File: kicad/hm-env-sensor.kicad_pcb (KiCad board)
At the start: 2 copper layers, 40 x 79 mm, 65 parts, among them Q1 Q12MHz/20pF/10ppm/4P/3.2x2.5mm, Q2 BC817-40(SOT23), Q3 BC817-40(SOT23), U1 BL4054B-42TPRN(SOT23-5), U2 CH340T(SSOP20W), U3 SY8089AAAC(SOT23-5), U4 BAT54C(SOT23-3), U5 ESP-WROOM-32, U6 BQ27441-G1, U7 BME280

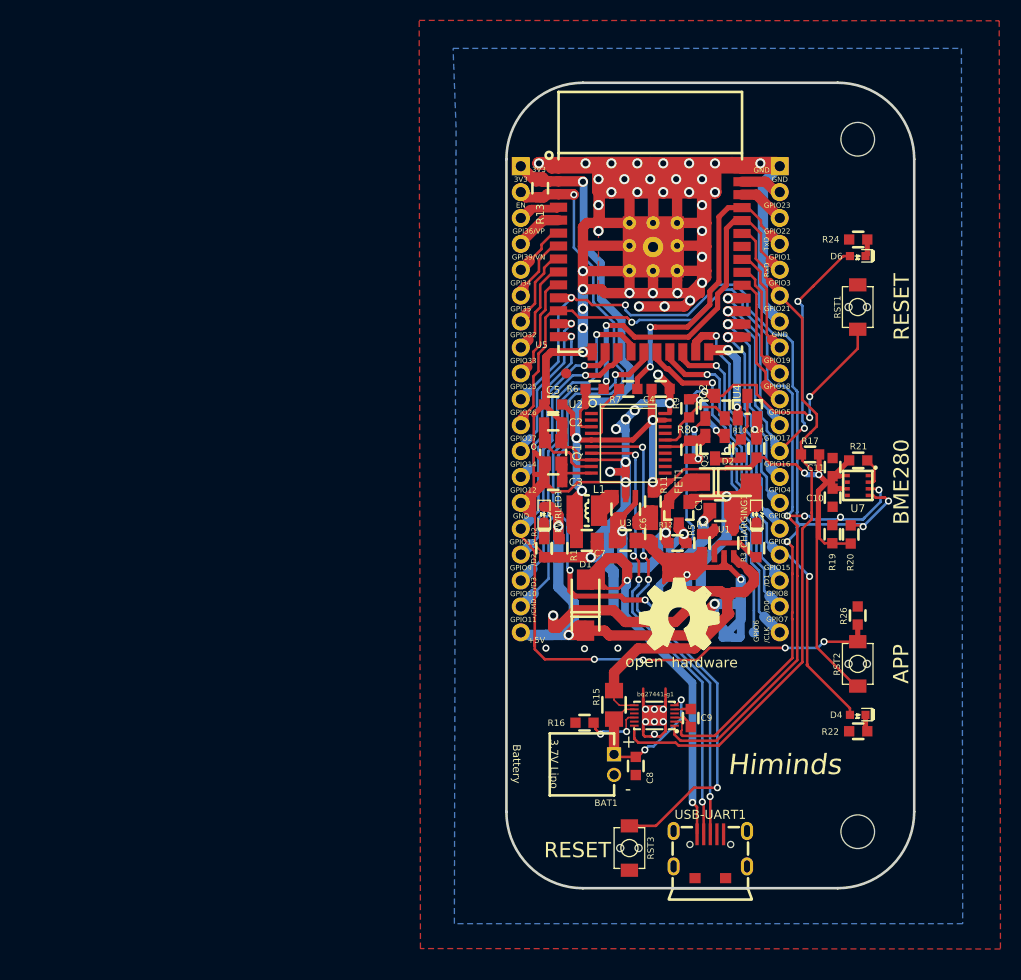
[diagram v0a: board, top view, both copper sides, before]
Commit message: Rev B updates
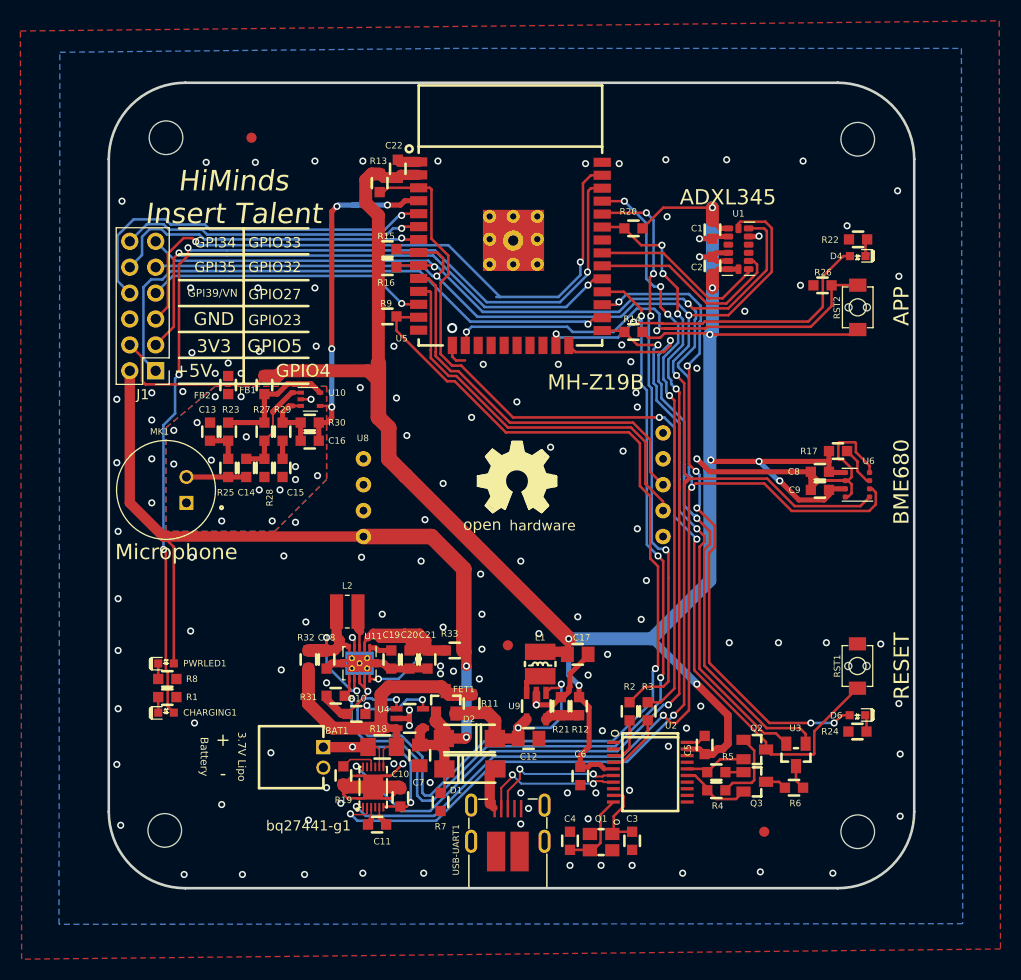
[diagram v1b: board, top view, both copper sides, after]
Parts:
- removed the ? at (146.3, 116.8)
- removed D_Com1, GND1: TESTPAD, OLIMEX_Other-FP:TESTPAD_40-ROUND
- removed EXT1, EXT2: HN1x19, OLIMEX_Connectors-FP:HN1x19
- removed RST3: IT-1185AU2-160G-G-TR, OLIMEX_Buttons-FP:IT1185AU2_V2
- added ?: , hm-env-sensor:LOGO_OPENHARDWARE_8x8, F.Cu at (130.4, 103.4)
- added C12: 47uF/6.3V/20%/X5R/C0805, OLIMEX_RLC-FP:C_0805_5MIL_DWS, F.Cu at (131.6, 128.5)
- added C13: 100nF/50V/20%/Y5V/C0603, OLIMEX_RLC-FP:C_0603_5MIL_DWS, F.Cu at (100.3, 98.4)
- added C14: 10nF/50V/20%/Y5V/C0603, OLIMEX_RLC-FP:C_0603_5MIL_DWS, F.Cu at (103.9, 102.0)
- added C15: 10uF/C0603, OLIMEX_RLC-FP:C_0603_5MIL_DWS, F.Cu at (107.4, 102.0)
- added C16: 100pF/C0603, OLIMEX_RLC-FP:C_0603_5MIL_DWS, F.Cu at (110.1, 99.3)
- added C17: 47uF/6.3V/20%/X5R/C0805, OLIMEX_RLC-FP:C_0805_5MIL_DWS, F.Cu at (136.4, 120.3)
- added C18: 10uF/6.3V/X7R/C0603, OLIMEX_RLC-FP:C_0603_5MIL_DWS, F.Cu at (111.8, 120.8)
- added C19: 1uF/6.3V/X7R/C0603, OLIMEX_RLC-FP:C_0603_5MIL_DWS, F.Cu at (118.1, 120.8)
- added C20: 10uF/6.3V/X7R/C0603, OLIMEX_RLC-FP:C_0603_5MIL_DWS, F.Cu at (119.9, 120.8)
- added C21: 10uF/6.3V/X7R/C0603, OLIMEX_RLC-FP:C_0603_5MIL_DWS, F.Cu at (121.7, 120.8)
- added C22: 10uF/6.3V/X7R/C0603, OLIMEX_RLC-FP:C_0603_5MIL_DWS, F.Cu at (118.7, 72.6)
- added FB1: Ferrite_Bead_Small, OLIMEX_RLC-FP:L_0603_5MIL_DWS, F.Cu at (105.7, 93.9)
- added FB2: Ferrite_Bead_Small, OLIMEX_RLC-FP:L_0603_5MIL_DWS, F.Cu at (102.1, 93.9)
- added FID1: Fiducial, OLIMEX_Other-FP:Fiducial1x3, F.Cu at (104.4, 69.6)
- added FID2: Fiducial, OLIMEX_Other-FP:Fiducial1x3, F.Cu at (154.7, 137.7)
- added J1: Conn_02x06_Odd_Even, Connector_PinHeader_2.54mm:PinHeader_2x06_P2.54mm_Vertical, F.Cu at (95.0, 92.5)
- added L2: LPS3015-222ML, Inductor_SMD:L_Wuerth_MAPI-3015, F.Cu at (113.8, 116.1)
- added MK1: Microphone, hm-env-sensor:MIC_CMA-4544PF-W, F.Cu at (96.0, 104.1)
- added MountingHole*: Mounting_hole_3.3mm, OLIMEX_Other-FP:Mounting_hole_3.3mm, F.Cu at (98.9, 56.0)
- added MountingHole*: Mounting_hole_3.3mm, OLIMEX_Other-FP:Mounting_hole_3.3mm, F.Cu at (98.8, 124.0)
- added R18: 0.01/1%/R1206, OLIMEX_RLC-FP:R_1206_5MIL_DWS, F.Cu at (117.2, 129.3)
- added R23: 1k/R0603, OLIMEX_RLC-FP:R_0603_5MIL_DWS, F.Cu at (102.1, 98.4)
- added R25: 1k/R0603, OLIMEX_RLC-FP:R_0603_5MIL_DWS, F.Cu at (102.1, 102.0)
- added R27: 1M/R0603, OLIMEX_RLC-FP:R_0603_5MIL_DWS, F.Cu at (105.7, 98.4)
- added R28: 1M/R0603, OLIMEX_RLC-FP:R_0603_5MIL_DWS, F.Cu at (105.7, 102.0)
- added R29: 1k/R0603, OLIMEX_RLC-FP:R_0603_5MIL_DWS, F.Cu at (107.4, 98.4)
- added R30: 20k/R0603, OLIMEX_RLC-FP:R_0603_5MIL_DWS, F.Cu at (110.1, 97.5)
- added R31: 10k, OLIMEX_RLC-FP:R_0603_5MIL_DWS, F.Cu at (112.6, 124.3)
- added R32: NA/R0603, OLIMEX_RLC-FP:R_0603_5MIL_DWS, F.Cu at (110.0, 120.8)
- added R33: NA/R0603, OLIMEX_RLC-FP:R_0603_5MIL_DWS, F.Cu at (124.3, 119.9)
- added U10: MAX4466, Package_TO_SOT_SMD:SOT-353_SC-70-5, F.Cu at (110.2, 95.2)
- added U11: TPS61202DRC, Package_SON:Texas_S-PVSON-N10_ThermalVias, F.Cu at (115.0, 121.1)
- added U8: MH-Z19B, hm-env-sensor:MH-Z19B, F.Cu at (130.0, 96.0)
- added U9: SY8089AAAC(SOT23-5), OLIMEX_Regulators-FP:SOT-23-5, F.Cu at (132.3, 125.3)
- C1: value 47uF/6.3V/20%/X5R/C0805 -> 4.7uF/50V/20%/Y5V/C0603; footprint OLIMEX_RLC-FP:C_0805_5MIL_DWS -> OLIMEX_RLC-FP:C_0603_5MIL_DWS
- C10: value 100nF/50V/20%/Y5V/C0603 -> 1.0uF/16V/10%/Y5V/C0603
- C11: value 100nF/50V/20%/Y5V/C0603 -> 0.47uF/50V/20%/Y5V/C0603
- C2: value 27pF/50V/5%/C0G/C0603 -> 100nF/50V/20%/Y5V/C0603
- C4: value 22uF/6.3V/20%/X5R/C0603 -> 27pF/50V/5%/C0G/C0603
- C5: value 100nF/50V/20%/Y5V/C0603 -> 22uF/6.3V/20%/X5R/C0603
- C6: value 47uF/6.3V/20%/X5R/C0805 -> 100nF/50V/20%/Y5V/C0603; footprint OLIMEX_RLC-FP:C_0805_5MIL_DWS -> OLIMEX_RLC-FP:C_0603_5MIL_DWS
- C8: value 1.0uF/16V/10%/Y5V/C0603 -> 100nF/50V/20%/Y5V/C0603
- C9: value 0.47uF/50V/20%/Y5V/C0603 -> 100nF/50V/20%/Y5V/C0603
- PWRLED1: value LED/RED/0603 -> LED/GREEN/0603
- R1: value 10k/R0603 -> 330/R0603
- R10: value 220R/R0603 -> 2.2k/R0603
- R11: value 4.99k/1%/R0603 -> NA/R0603
- R12: value 1.1k/1%/R0603 -> 4.99k/1%/R0603
- R15: value 0.01/1%/R1206 -> 4.7k/R0603; footprint OLIMEX_RLC-FP:R_1206_5MIL_DWS -> OLIMEX_RLC-FP:R_0603_5MIL_DWS
- R16: value 10k/R0603 -> 4.7k/R0603
- R19: value 4.7k/R0603 -> 10k/R0603
- R2, R3: value 2.2k/R0603 -> 220R/R0603
- R21: value 4.7k/R0603 -> 1.1k/1%/R0603
- R4: value 2.2k/R0603 -> 1k/R0603
- R5: value NA/R0603 -> 1k/R0603
- R7: value 220R/R0603 -> 10k/R0603
- R8: value 1k/R0603 -> 4.7k/R0603
- R9: value 1k/R0603 -> 10k/R0603
- U1: value BL4054B-42TPRN(SOT23-5) -> ADXL345; footprint OLIMEX_IC-FP:SOT-23-5 -> Package_LGA:LGA-14_3x5mm_P0.8mm_LayoutBorder1x6y
- U3: value SY8089AAAC(SOT23-5) -> BAT54C(SOT23-3); footprint OLIMEX_Regulators-FP:SOT-23-5 -> OLIMEX_Diodes-FP:SOT23-3
- U4: value BAT54C(SOT23-3) -> BL4054B-42TPRN(SOT23-5); footprint OLIMEX_Diodes-FP:SOT23-3 -> OLIMEX_IC-FP:SOT-23-5
- U6: value BQ27441-G1 -> BME680; footprint sparkfun-battery-babysitter:PDSO-N12 -> Package_LGA:Bosch_LGA-8_3x3mm_P0.8mm_ClockwisePinNumbering
- U7: value BME280 -> BQ27441-G1; footprint SparkFun_BME280_Breakout_v10:BME280_LGA -> hm-env-sensor:PDSO-N12
- USB-UART1: footprint OLIMEX_Connectors-FP:USB-MICRO_MISB-SWMM-5B_LF -> hm-env-sensor:USB_Micro_B_Male_UJ2-MIBH-4-SMT-TR
- moved CHARGING1 61.1 mm to (96.0, 126.0), turned to 0 degrees
- moved C11 56.8 mm to (116.7, 137.0), turned to 180 degrees
- moved U7 56.0 mm to (116.3, 133.3)
- moved R8 55.9 mm to (96.1, 122.7), turned to 180 degrees
- moved R19 53.5 mm to (113.4, 132.1), turned to 90 degrees
- moved C10 51.6 mm to (119.0, 134.3), turned to 90 degrees
- moved R15 49.9 mm to (117.7, 80.5), turned to 180 degrees
- moved R16 48.7 mm to (117.7, 82.3), turned to 180 degrees
- moved R24 48.3 mm to (163.8, 127.8)
- moved R22 48.2 mm to (163.9, 79.6)
- moved R10 45.8 mm to (114.7, 126.1), turned to 180 degrees
- moved C4 45.2 mm to (135.6, 138.6), turned to 90 degrees
- moved U4 45.1 mm to (119.9, 126.6), turned to 180 degrees
- moved D6 45.0 mm to (163.8, 126.2)
- moved D4 45.0 mm to (163.9, 81.2)
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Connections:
- net /+5V_USB renamed /Power and charger/+5V_USB
- net Net-(U2-Pad6) renamed /USB2UART/D+
- net Net-(U2-Pad7) renamed /USB2UART/D-
- BAT1 pad 1: /BATTERY_IN -> /BATTERY
- C1 pad 1: +5V -> +3V3
- C10 pad 1: +3V3 -> /BATTERY
- C11 pad 1: +3V3 -> Net-(C11-Pad1)
- C2 pad 1: Net-(C2-Pad1) -> +3V3
- C4 pad 1: +3V3 -> Net-(C4-Pad1)
- C6 pad 1: Net-(C6-Pad1) -> +3V3
- C7 pad 1: +3V3 -> +5V
- C8 pad 1: /BATTERY_IN -> +3V3
- C9 pad 1: Net-(C9-Pad1) -> +3V3
- CHARGING1 pad 2: +5V -> /GPIO22
- D2 pad 1: Net-(C6-Pad1) -> Net-(C12-Pad1)
- FET1 pad 2: Net-(C6-Pad1) -> Net-(C12-Pad1)
- FET1 pad 3: V_BATT -> /AFTER_BAT_SENSOR
- Q1 pad 1: Net-(C2-Pad1) -> Net-(C3-Pad1)
- Q1 pad 2: Net-(C3-Pad1) -> Net-(C4-Pad1)
- R1 pad 1: +5V -> GND
- R1 pad 2: GND -> Net-(CHARGING1-Pad1)
- R10 pad 1: Net-(Q3-Pad3) -> Net-(R10-Pad1)
- R10 pad 2: /D_Com -> GND
- R11 pad 1: Net-(R11-Pad1) -> /AFTER_BAT_SENSOR
- R11 pad 2: +3V3 -> Net-(C12-Pad1)
- R12 pad 1: Net-(R11-Pad1) -> Net-(R12-Pad1)
- R12 pad 2: GND -> +3V3
- R15 pad 1: V_BATT -> /GPIO32
- R15 pad 2: /BATTERY_IN -> +3V3
- R16 pad 1: GND -> /GPIO33
- R16 pad 2: Net-(R16-Pad2) -> +3V3
- R17 pad 1: /GPIO21 -> Net-(R17-Pad1)
- R19 pad 1: /GPIO27 -> GND
- R19 pad 2: +3V3 -> Net-(R19-Pad2)
- R2 pad 1: Net-(PWRLED1-Pad1) -> Net-(R2-Pad1)
- R2 pad 2: GND -> /GPIO3
- R20 pad 1: /GPIO26 -> /GPIO21
- R21 pad 1: Net-(R21-Pad1) -> Net-(R12-Pad1)
- R21 pad 2: +3V3 -> GND
- R3 pad 1: Net-(CHARGING1-Pad1) -> Net-(R3-Pad1)
- R3 pad 2: Net-(R3-Pad2) -> /GPIO1
- R4 pad 1: Net-(R4-Pad1) -> Net-(Q3-Pad2)
- R4 pad 2: GND -> Net-(Q2-Pad1)
- R5 pad 1: V_BATT -> Net-(Q2-Pad2)
- R5 pad 2: Net-(C6-Pad1) -> Net-(Q3-Pad1)
- R6 pad 1: Net-(R6-Pad1) -> Net-(Q3-Pad3)
- R6 pad 2: /GPIO3/U0RXD -> Net-(R6-Pad2)
- R7 pad 1: Net-(R7-Pad1) -> +5V
- R7 pad 2: /GPIO1/U0TXD -> GND
- R8 pad 1: Net-(Q3-Pad2) -> GND
- R8 pad 2: Net-(Q2-Pad1) -> Net-(PWRLED1-Pad1)
- R9 pad 1: Net-(Q2-Pad2) -> +3V3
- R9 pad 2: Net-(Q3-Pad1) -> /GPIO14
- U1 pad 1: Net-(R3-Pad2) -> +3V3
- U1 pad 3: V_BATT -> Net-(U1-Pad3)
- U1 pad 4: +5V -> GND
- U1 pad 5: Net-(R4-Pad1) -> GND
- U2 pad 10: Net-(C3-Pad1) -> Net-(C4-Pad1)
- U2 pad 3: Net-(R6-Pad1) -> Net-(R2-Pad1)
- U2 pad 4: Net-(R7-Pad1) -> Net-(R3-Pad1)
- U2 pad 9: Net-(C2-Pad1) -> Net-(C3-Pad1)
- U3 pad 1: Net-(C6-Pad1) -> /GPIO2
- U3 pad 2: GND -> /GPIO0
- U3 pad 3: Net-(L1-Pad1) -> Net-(R6-Pad2)
- U4 pad 1: /GPIO2 -> /GPIO14
- U4 pad 2: /GPIO0 -> GND
- U4 pad 3: /D_Com -> /AFTER_BAT_SENSOR
- U5 pad 14: /GPIO12 -> Net-(U5-Pad14)
- U5 pad 17: /GPIO9/SD_DATA2 -> Net-(U5-Pad17)
- U5 pad 18: /GPIO10/SD_DATA3 -> Net-(U5-Pad18)
- U5 pad 19: /GPIO11/SD_CMD -> Net-(U5-Pad19)
- U5 pad 20: /GPIO6/SD_CLK -> Net-(U5-Pad20)
- U5 pad 21: /GPIO7/SD_DATA0 -> Net-(U5-Pad21)
- U5 pad 22: /GPIO8/SD_DATA1 -> Net-(U5-Pad22)
- U5 pad 34: /GPIO3/U0RXD -> /GPIO3
- U5 pad 35: /GPIO1/U0TXD -> /GPIO1
- U5 pad 4: /GPI36/SENSOR_VP -> /GPI36
- U5 pad 5: /GPI39/SENSOR_VN -> /GPI39
- U6 pad 1: /GPIO27 -> GND
- U6 pad 2: /GPIO26 -> Net-(R17-Pad1)
- U6 pad 3: GND -> /GPIO33
- U6 pad 4: (no net) -> /GPIO32
- U6 pad 5: Net-(C9-Pad1) -> GND
- U6 pad 6: /BATTERY_IN -> +3V3
- U6 pad 7: V_BATT -> GND
- U6 pad 8: /BATTERY_IN -> +3V3
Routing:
- net GND: track 438.5 -> 99.3 mm, vias 59 -> 130
- net /GPIO32: track 9.13 -> 180.6 mm, vias 0 -> 5
- net /GPIO33: track 9.26 -> 176.5 mm, vias 0 -> 5
- net +3V3: track 146.7 -> 252.4 mm, vias 7 -> 9
- net /GPIO22: track 4.65 -> 99.2 mm, vias 0 -> 4
- net /GPIO14: track 15.8 -> 103.1 mm, vias 1 -> 2
- net /GPIO27: track 104.0 -> 27.6 mm, vias 5 -> 1
- net /GPIO17: track 15.9 -> 88.9 mm, vias 1 -> 4
- net /GPIO26: track 103.2 -> 39.6 mm, vias 5 -> 0
- net /GPIO23: track 4.12 -> 63.0 mm, vias 0 -> 2
- net /GPIO1: track 0.00 -> 56.8 mm, vias 0 -> 4
- net /GPIO3: track 0.00 -> 56.7 mm, vias 0 -> 4
- net V_BATT: track 53.4 -> 0.00 mm, vias 2 -> 0
- net /ESP_EN: track 142.0 -> 97.5 mm, vias 7 -> 2
- net /GPIO5: track 13.1 -> 54.8 mm, vias 0 -> 2
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- added copper zone on B.Cu, net GNDA
- added copper zone on F.Cu, net GNDA
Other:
- board size 40 x 79 mm -> 79 x 79 mm
- board text added: "ADXL345"
- board text added: "BME680"
- board text added: "HiMinds Insert Talent"
- board text added: "MH-Z19B"
- board text added: "Microphone"
- board text added: "hw-env-sensor Rev.B"
- board text removed: "/CLK"
- board text removed: "/CMD"
- board text removed: "/D0"
- board text removed: "/D1"
- board text removed: "/D2"
- board text removed: "/D3"
- board text removed: "BME280"
- board text removed: "EN"
- board text removed: "ESP_EN"
- board text removed: "GPI36/VP"
- board text removed: "GPIO0"
- board text removed: "GPIO1"
- board text removed: "GPIO1/ U0TXD"
- board text removed: "GPIO10"
- board text removed: "GPIO10/ SD_DATA3"
- board text removed: "GPIO11"
- board text removed: "GPIO11/ SD_CMD"
- board text removed: "GPIO12"
- board text removed: "GPIO13"
- board text removed: "GPIO14"
- board text removed: "GPIO15"
- board text removed: "GPIO16"
- board text removed: "GPIO17"
- board text removed: "GPIO18"
- board text removed: "GPIO19"
- board text removed: "GPIO2"
- board text removed: "GPIO21"
- board text removed: "GPIO22"
- board text removed: "GPIO25"
- board text removed: "GPIO26"
- board text removed: "GPIO3"
- board text removed: "GPIO3/ U0RXD"
- board text removed: "GPIO6"
- board text removed: "GPIO6/ SD_CLK"
- board text removed: "GPIO7"
- board text removed: "GPIO7/ SD_DATA0"
- board text removed: "GPIO8"
- board text removed: "GPIO8/ SD_DATA1"
- board text removed: "GPIO9"
- board text removed: "GPIO9/ SD_DATA2"
- board text removed: "Himinds"
- board text removed: "RxD"
- board text removed: "TxD"
- board text removed: "hw-env-sensor Rev.A"
